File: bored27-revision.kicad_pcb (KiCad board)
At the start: 2 copper layers, 195.3 x 78.6 mm, 73 parts, among them J1 USB_C_Receptacle_USB2.0, J2 AVR-ISP-6, K1 Q, K10 P, K11 A, K12 S, K13 D, K14 F, K15 G, K16 H, K17 J, K18 K, K19 L, K2 W, K20 Z, K21 X, K22 C, K23 V, K24 B, K25 N, K26 M, K27 SPACE, K3 E, K4 R, K5 T, K6 Y, K7 U, K8 I, K9 O, SW1 SW_Push, U1 ATmega32U2-A, U2 PRTR5V0U2X, X1 16MHz

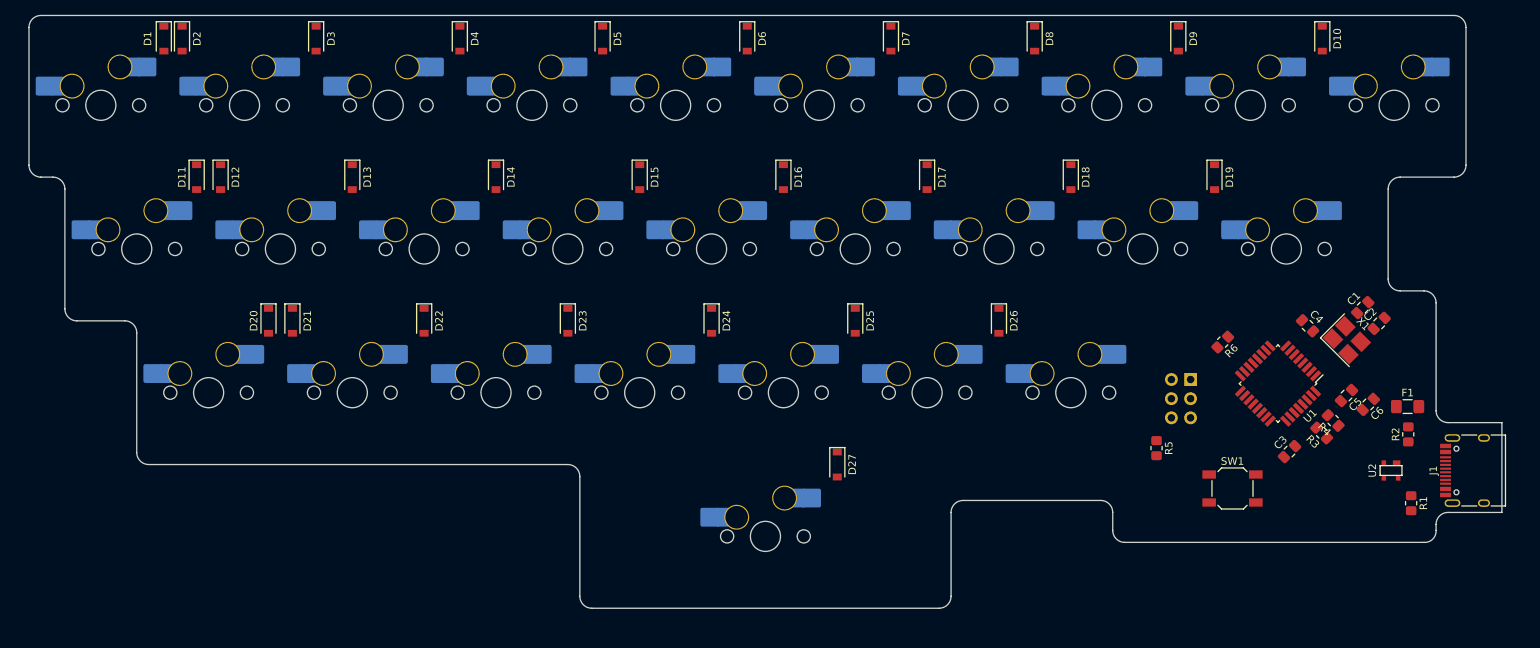
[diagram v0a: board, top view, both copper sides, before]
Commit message: finished pcb
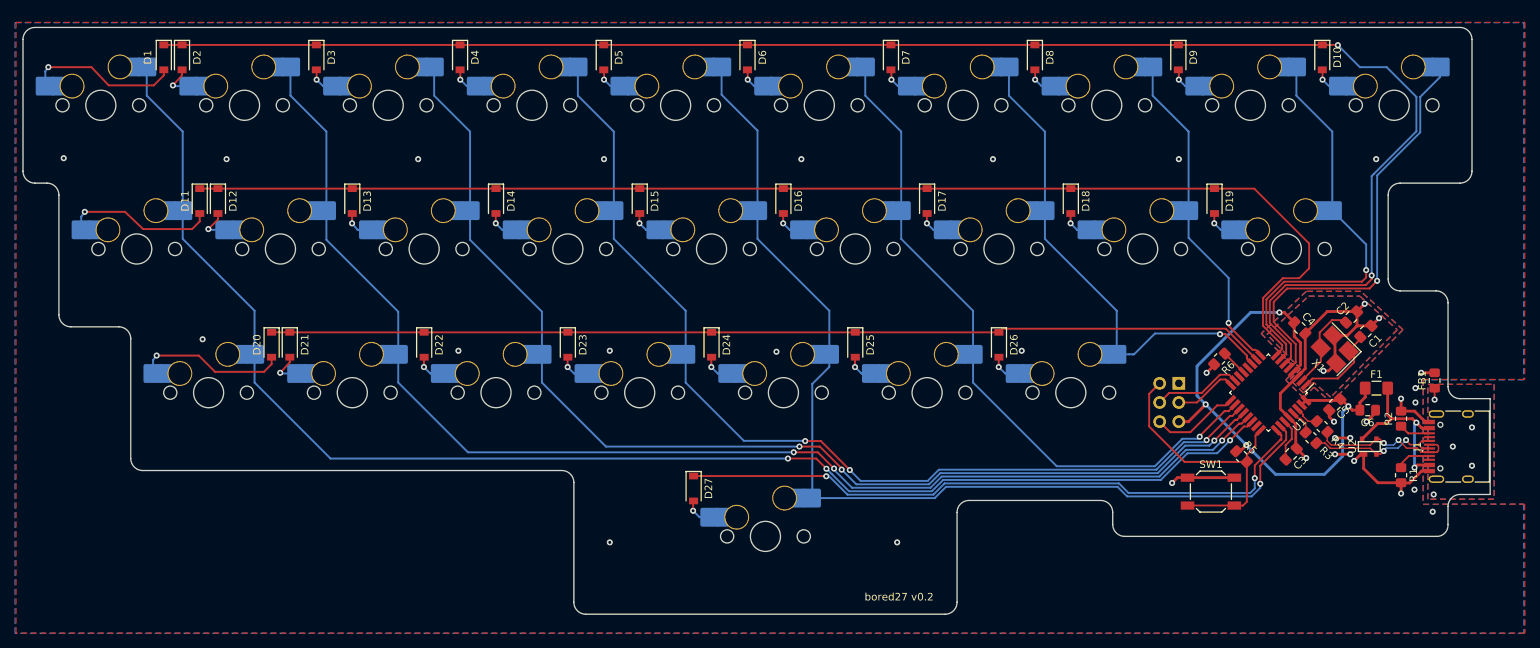
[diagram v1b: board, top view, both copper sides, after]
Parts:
- added FB1: 60@100MHz, Inductor_SMD:L_0805_2012Metric_Pad1.15x1.40mm_HandSolder, F.Cu at (236.3, 105.5)
- moved D27 19.3 mm to (138.1, 119.9)
- moved R5 11.3 mm to (210.7, 115.6), turned to -45 degrees
- moved F1 4.80 mm to (228.6, 106.6)
- moved U2 4.29 mm to (227.7, 114.3), turned to 90 degrees
- moved R1 3.95 mm to (231.9, 118.1)
- moved J1 3.82 mm to (239.7, 114.3)
- moved C2 3.77 mm to (225.3, 97.1)
- moved D20 3.20 mm to (82.2, 100.8)
- moved D11 3.20 mm to (72.6, 81.8)
- moved D21 3.19 mm to (84.6, 100.8)
- moved D12 3.19 mm to (75.1, 81.8)
- moved C1 3.18 mm to (227.2, 99.0)
- moved D22 3.18 mm to (102.4, 100.8)
- moved D23 3.18 mm to (121.4, 100.8)
- moved D24 3.18 mm to (140.5, 100.8)
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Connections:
- J1 pad A6: D+ -> DP
- J1 pad A7: D- -> DN
- J1 pad B6: D+ -> DP
- J1 pad B7: D- -> DN
- J1 pad S1: GND -> Earth
- R3 pad 1: D+ -> DP
- R3 pad 2: Net-(R3-Pad2) -> D+
- R4 pad 1: D- -> DN
- R4 pad 2: Net-(R4-Pad2) -> D-
- U1 pad 10: unconnected-(U1-Pad10) -> ROW2
- U1 pad 11: unconnected-(U1-Pad11) -> COL6
- U1 pad 14: ROW0 -> unconnected-(U1-Pad14)
- U1 pad 18: ROW1 -> COL5
- U1 pad 19: ROW2 -> COL3
- U1 pad 20: ROW3 -> COL2
- U1 pad 21: COL0 -> COL1
- U1 pad 22: COL5 -> COL0
- U1 pad 23: COL4 -> unconnected-(U1-Pad23)
- U1 pad 25: COL3 -> ROW3
- U1 pad 26: COL2 -> COL4
- U1 pad 29: Net-(R3-Pad2) -> D+
- U1 pad 30: Net-(R4-Pad2) -> D-
- U1 pad 5: COL1 -> COL9
- U1 pad 6: COL6 -> ROW0
- U1 pad 7: COL7 -> COL8
- U1 pad 8: COL8 -> ROW1
- U1 pad 9: COL9 -> COL7
- U2 pad 2: D+ -> DP
- U2 pad 3: D- -> DN
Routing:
- net ROW0: track 0.00 -> 220.0 mm, vias 0 -> 2
- net COL0: track 0.00 -> 189.8 mm, vias 0 -> 3
- net COL1: track 0.00 -> 170.1 mm, vias 0 -> 3
- net ROW1: track 0.00 -> 170.1 mm
- net COL2: track 0.00 -> 150.4 mm, vias 0 -> 3
- net COL4: track 0.00 -> 135.1 mm, vias 0 -> 1
- net ROW2: track 0.00 -> 132.4 mm
- net COL3: track 0.00 -> 130.6 mm, vias 0 -> 3
- net COL5: track 0.00 -> 90.5 mm, vias 0 -> 1
- net ROW3: track 0.00 -> 86.4 mm, vias 0 -> 2
- net GND: track 0.00 -> 84.6 mm, vias 0 -> 36
- net +5V: track 0.00 -> 77.2 mm, vias 0 -> 4
- net COL6: track 0.00 -> 65.0 mm, vias 0 -> 1
- net COL9: track 0.00 -> 57.1 mm, vias 0 -> 1
- net COL8: track 0.00 -> 55.5 mm, vias 0 -> 1
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- added copper zone on B.Cu, net Earth
- added copper zone on F.Cu, net Earth
- added copper zone on B.Cu, net GND
- added copper zone on F.Cu, net GND
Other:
- board size 195.3 x 78.6 mm -> 194.5 x 77.8 mm
- board text added: "bored27 v0.2"
